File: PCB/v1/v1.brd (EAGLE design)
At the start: 81.5 x 40.5 mm, 64 parts, among them U2 AT24C512C-SHD-B

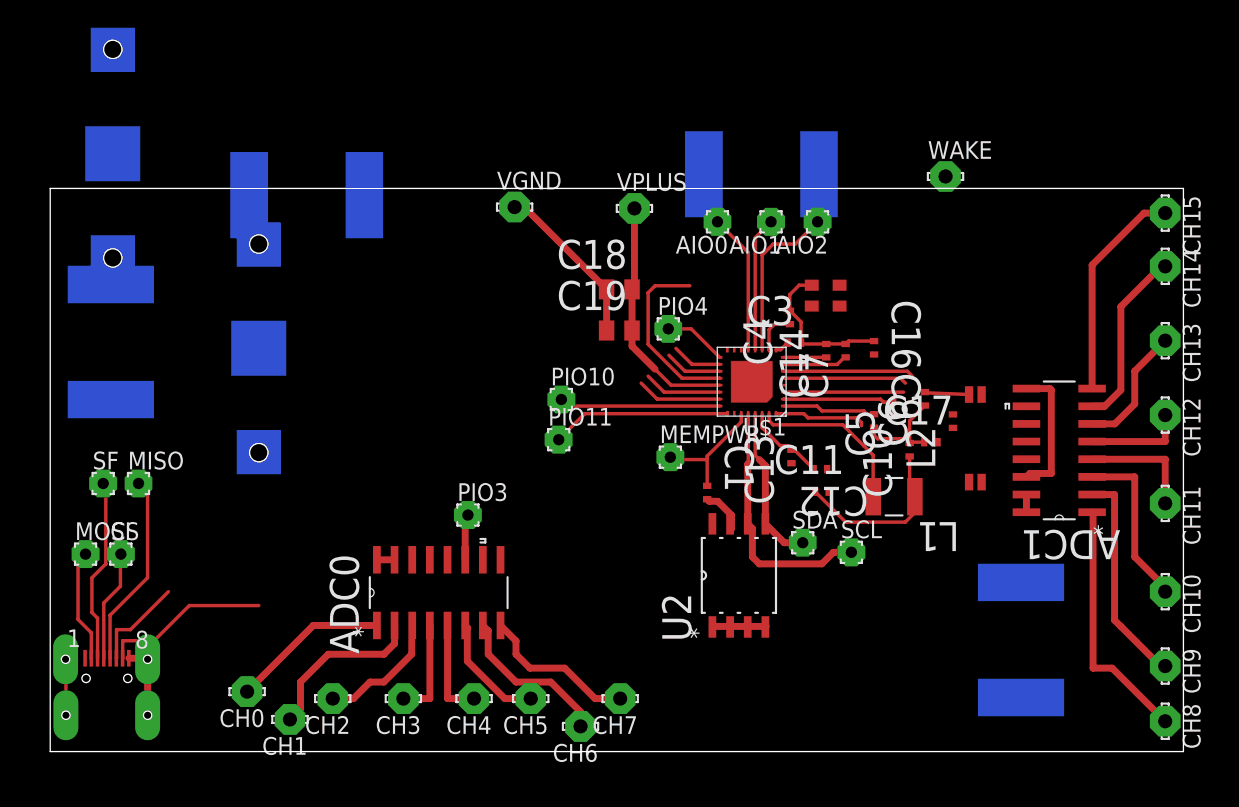
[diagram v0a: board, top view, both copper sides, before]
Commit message: push to work from main pc
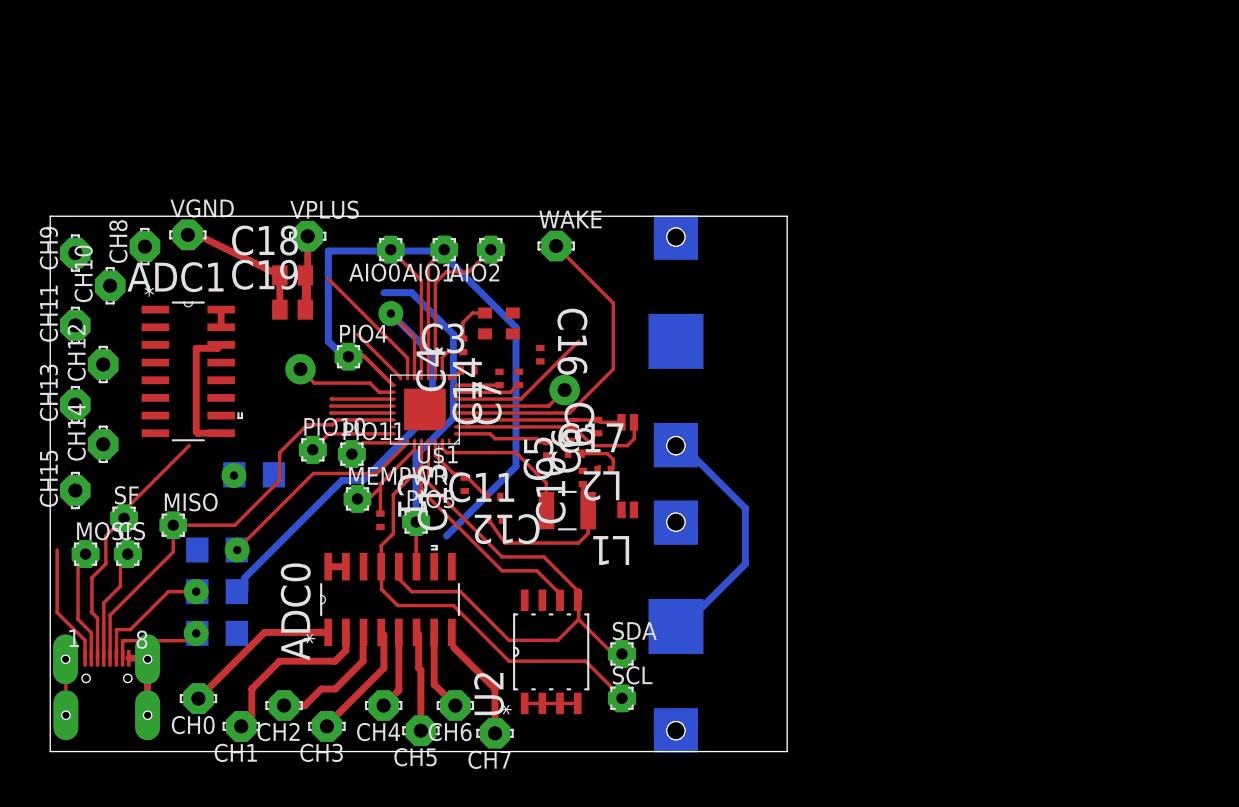
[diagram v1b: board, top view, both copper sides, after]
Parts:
- removed R1, R2, R3, R4: (no value), resistor-shunt:BVS
- added R5, R6, R7, R8: (no value), eagle-ltspice:R1206
- moved CH9 83.8 mm to (1.81, 35.9), turned to 90 degrees
- moved CH8 80.9 mm to (6.81, 36.3), turned to 90 degrees
- moved CH15 80.9 mm to (1.81, 18.8), turned to 90 degrees
- moved CH11 79.4 mm to (1.81, 30.6), turned to 90 degrees
- moved CH10 79.0 mm to (4.31, 33.5), turned to 90 degrees
- moved CH13 78.5 mm to (1.81, 24.9), turned to 90 degrees
- moved CH14 77.4 mm to (3.81, 22.1), turned to 90 degrees
- moved CH12 76.5 mm to (3.81, 27.8), turned to 90 degrees
- moved ADC1 62.9 mm to (9.93, 27.3), turned to 0 degrees
- moved U$5 52.9 mm to (45.0, 9.00), turned to 90 degrees
- moved U$6 30.0 mm to (45.0, 29.5), turned to 90 degrees
- moved WAKE 28.4 mm to (36.4, 36.4)
- moved L2 27.3 mm to (37.7, 21.4), turned to 180 degrees
- moved U$4 25.1 mm to (40.8, 23.1)
- moved C16 24.0 mm to (35.2, 28.5)
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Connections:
- net N$20: now also R7.1; no longer R1.2
- net N$36: now also R6.1; no longer R2.2
- net N$37: now also R7.2; no longer R1.1
- net N$38: now also R6.2; no longer R2.1
- net N$40: now also R8.1; no longer R4.2
- net N$45: now also R5.1; no longer R3.1
- net VDD: now also R5.2, R8.2; no longer R3.2, R4.1
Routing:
- net N$25: track 4.55 -> 49.4 mm
- net N$37: track 0.00 -> 33.6 mm
- net N$21: track 18.2 -> 47.1 mm
- net N$22: track 11.5 -> 39.5 mm
- net N$23: track 3.30 -> 28.5 mm
- net GND: track 62.9 -> 39.4 mm
- net N$49: track 0.00 -> 23.1 mm
- net N$16: track 18.0 -> 0.00 mm
- net N$48: track 0.00 -> 17.7 mm
- net N$9: track 15.7 -> 0.00 mm
- net N$15: track 15.7 -> 0.00 mm
- net N$45: track 0.00 -> 15.6 mm
- net N$10: track 12.8 -> 0.00 mm
- net N$14: track 12.2 -> 0.00 mm
- net N$18: track 19.8 -> 31.6 mm
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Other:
- board size 81.5 x 40.5 mm -> 53 x 38.5 mm

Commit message: takes its time
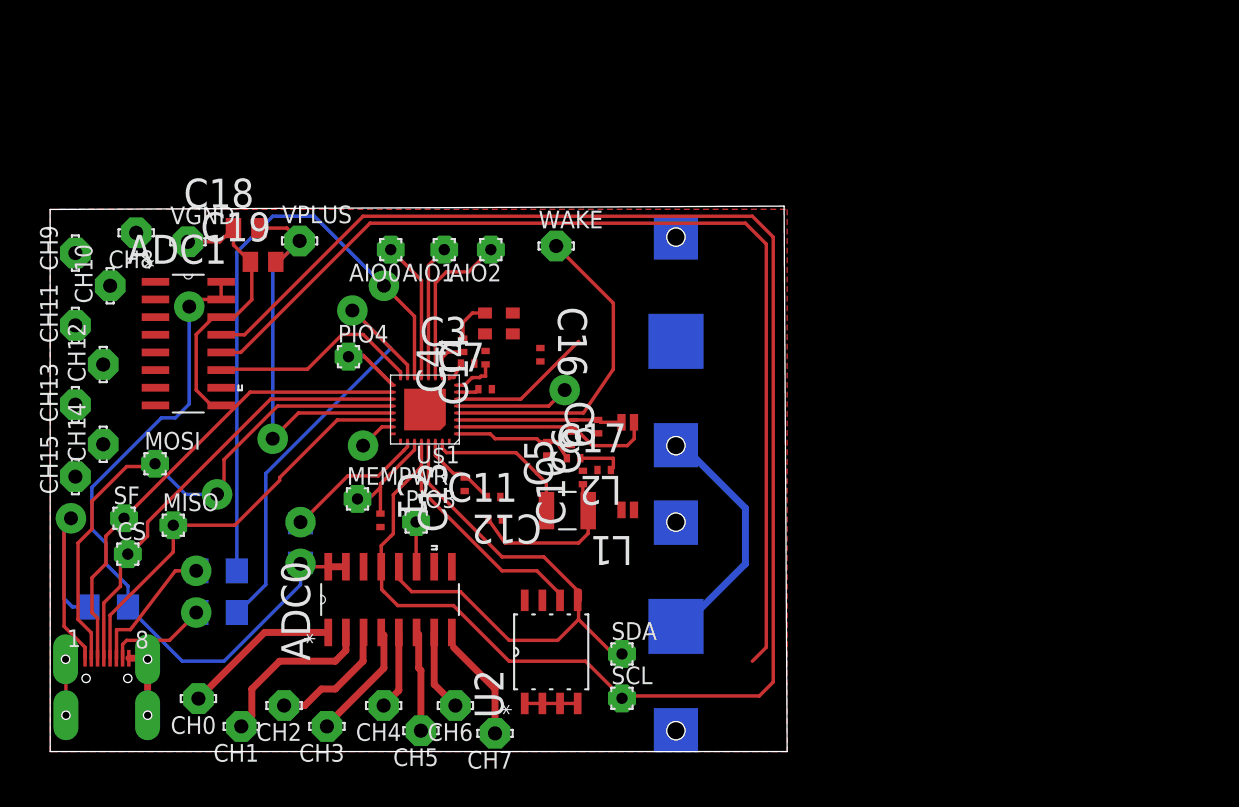
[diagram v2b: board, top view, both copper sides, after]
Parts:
- removed PIO10, PIO11: (no value), wirepad:1,6/0,8
- moved R8 14.2 mm to (4.17, 10.4)
- moved MOSI 8.20 mm to (7.54, 20.7)
- moved R5 6.02 mm to (18.0, 15.0), turned to 270 degrees
- moved C18 4.77 mm to (14.1, 37.6)
- moved C19 4.04 mm to (15.3, 35.2)
- moved C7 2.55 mm to (31.3, 26.1), turned to 0 degrees
- moved ADC1 2.00 mm to (9.93, 29.3)
- moved C14 1.80 mm to (31.3, 28.3)
- moved R6 1.50 mm to (12.0, 10.0)
- moved R7 1.50 mm to (12.0, 13.0)
- moved CH8 1.17 mm to (6.18, 37.3), turned to 180 degrees
- moved CH15 1.00 mm to (1.81, 19.8)
- moved VPLUS 0.67 mm to (17.9, 36.7)
- moved C3 0.50 mm to (30.0, 27.9)
- moved VGND 0.50 mm to (9.90, 36.7)
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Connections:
- removed net N$42: PIO10.1, U$1.PIO[10]
- removed net N$47: PIO11.1, U$1.PIO[11]
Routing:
- net N$21: track 47.1 -> 134.0 mm
- net N$22: track 39.5 -> 113.6 mm
- net VDD: track 2.56 -> 51.2 mm, vias 0 -> 1
- net N$25: track 49.4 -> 8.09 mm
- net N$50: track 12.6 -> 39.6 mm, vias 0 -> 1
- net N$38: track 9.46 -> 34.4 mm
- net N$31: track 12.6 -> 32.5 mm
- net N$34: track 18.7 -> 33.4 mm, vias 0 -> 1
- net N$37: track 33.6 -> 44.2 mm, vias 0 -> 1
- net N$40: track 8.90 -> 19.3 mm
- net N$23: track 28.5 -> 18.7 mm
- net N$51: track 25.7 -> 34.3 mm
- net N$42: track 6.24 -> 0.00 mm, vias 0 -> 1
- net N$45: track 15.6 -> 10.4 mm
- net N$47: track 3.94 -> 0.00 mm, vias 0 -> 1
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- added copper zone on layer 1, net GND
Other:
- board size 53 x 38.5 mm -> 53 x 39.2 mm

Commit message: getting there
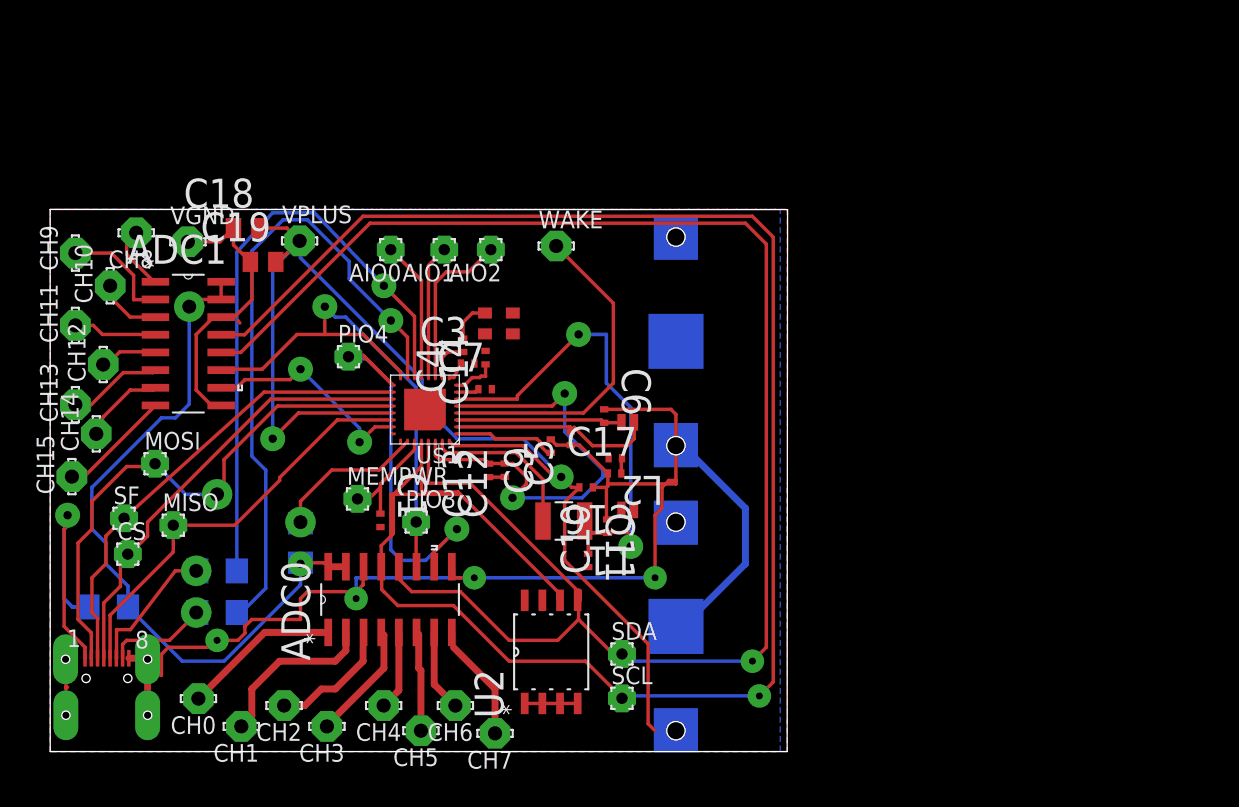
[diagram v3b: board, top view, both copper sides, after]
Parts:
- moved C16 10.1 mm to (38.5, 19.0), turned to 180 degrees
- moved C11 7.31 mm to (38.7, 13.8), turned to 270 degrees
- moved C10 3.91 mm to (40.1, 16.2)
- moved L2 3.00 mm to (40.6, 21.1)
- moved C12 2.08 mm to (32.7, 20.2), turned to 90 degrees
- moved C13 2.02 mm to (31.6, 20.2)
- moved CH14 0.90 mm to (3.31, 22.9)
- moved C6 0.88 mm to (39.8, 24.1), turned to 270 degrees
- moved C17 0.79 mm to (40.6, 20.0)
- moved L1 0.79 mm to (36.9, 16.6)
- moved C9 0.31 mm to (36.0, 22.0), turned to 90 degrees
- moved CH15 0.25 mm to (1.56, 19.8)
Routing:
- net GND: track 37.1 -> 118.8 mm, vias 0 -> 4
- net N$34: track 33.4 -> 93.1 mm, vias 1 -> 2
- net N$25: track 8.09 -> 33.4 mm, vias 0 -> 1
- net N$23: track 18.7 -> 39.4 mm, vias 0 -> 1
- net N$28: track 14.2 -> 32.5 mm, vias 0 -> 2
- net N$39: track 23.7 -> 37.8 mm, vias 0 -> 2
- net N$24: track 2.71 -> 16.1 mm, vias 0 -> 2
- net N$38: track 34.4 -> 46.7 mm, vias 0 -> 1
- net N$22: track 113.6 -> 123.2 mm, vias 0 -> 1
- net N$21: track 134.0 -> 143.0 mm, vias 0 -> 1
- net N$15: track 0.00 -> 8.18 mm
- net N$9: track 0.00 -> 8.13 mm
- net N$11: track 0.00 -> 6.79 mm
- net N$13: track 0.00 -> 6.04 mm
- net N$10: track 0.00 -> 5.94 mm
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- added copper zone on layer 16, net GND
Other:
- board size 53 x 39.2 mm -> 53 x 39 mm
